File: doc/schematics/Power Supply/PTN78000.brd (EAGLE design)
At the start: 160 x 100 mm, 5 parts, among them U1 1.5APOWERMODULE

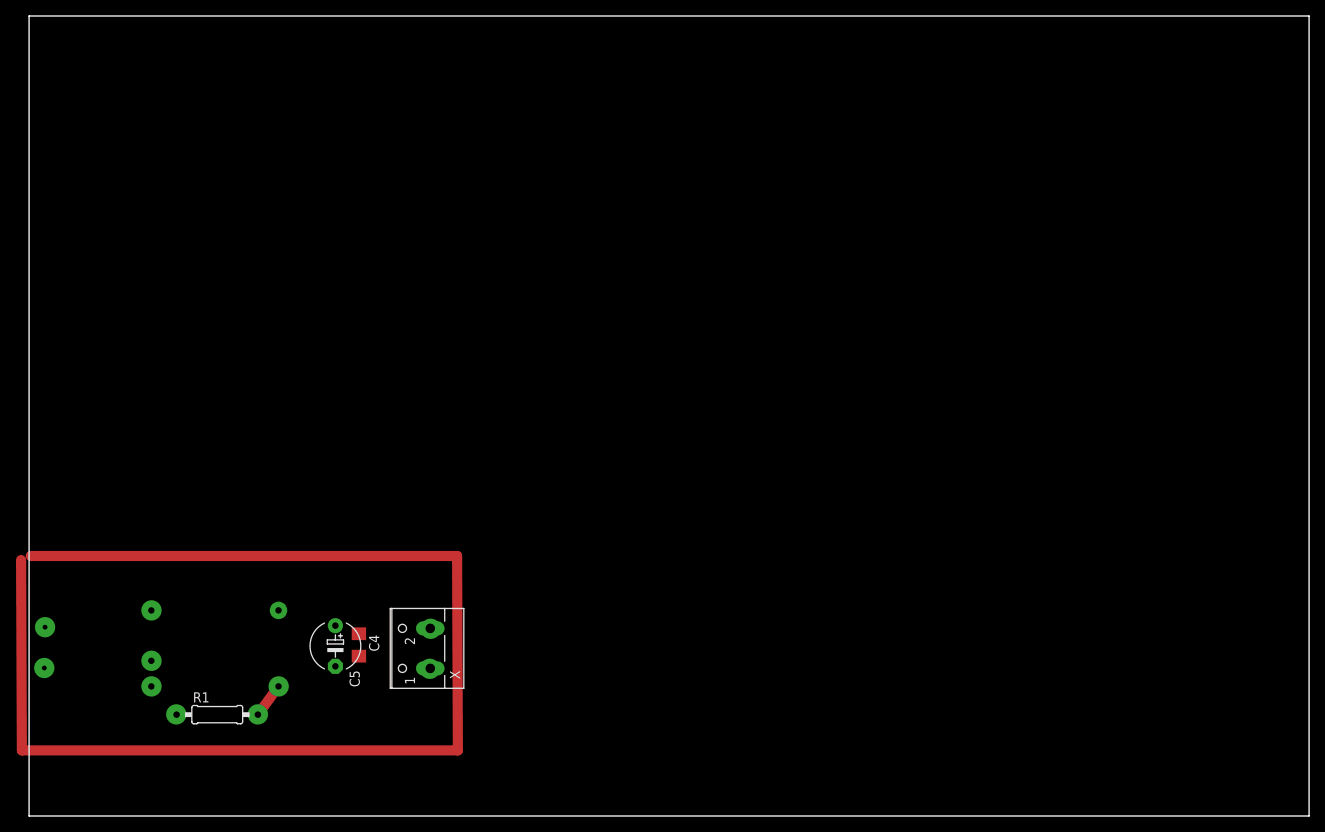
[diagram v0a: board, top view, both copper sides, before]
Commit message: New schematics
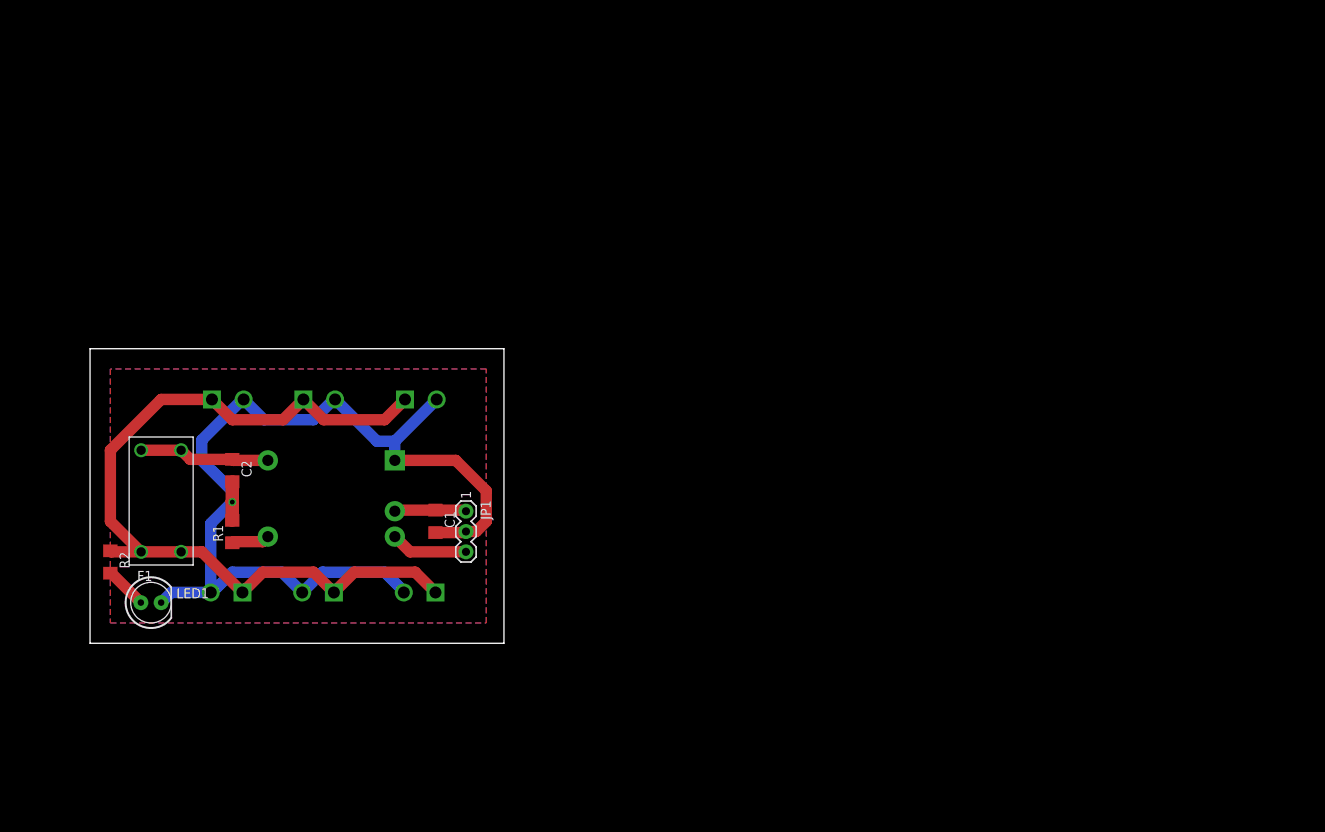
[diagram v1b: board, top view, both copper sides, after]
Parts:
- removed C4: (no value), rcl:C1206
- removed C5: (no value), rcl:E5-6
- removed U1: 1.5APOWERMODULE, TIPOWERMODULE:1.5APOWERMODULE
- removed X: OUTPUT (6 V), con-wago-500:W237-102
- added C1: 2.2 uF, ASL:1206
- added C2: 100 uF, ASL:1206
- added F1: FUSE, ASL:FUSE_2AG
- added J11, J13, J14, J15, J16, J9: POW_CONNECTFEMALE-RA, ASL:SOCKET-FEMALE_RA-3.96MM-2
- added JP1: M03PTH, ASL:1X03
- added LED1: (no value), SparkFun-LED:LED5MM
- added R2: 330, ASL:1206
- added U$1: PTN78000THROUGH-HOLE, ASL:PTN78000
- R1: value 13.1 K -> 21 K; device rcl:0207/10 -> ASL:1206
- moved R1 23.0 mm to (25.4, 35.6), turned to 90 degrees
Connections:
- removed net VCC: U1.P$2
- new net N$4: JP1.3, U$1.INHIBIT
- new net N$5: C2.1, F1.P$1, F1.P$2, U$1.V_OUT
- new net N$6: LED1.A, R2.2
- new net VCC5V0: F1.P$3, F1.P$4, J11.1, J13.1, J14.1, J15.1, J16.1, J9.1, R2.1
- net GND: now also C1.2, C2.2, J11.2, J13.2, J14.2, J15.2, J16.2, J9.2, JP1.2, LED1.K, R1.2, U$1.GND; no longer C4.2, C5.-, R1.1, U1.P$1
- net N$1: now also C1.1, JP1.1, U$1.V_IN; no longer R1.2, U1.P$4
- net N$2: now also R1.1, U$1.ADJ; no longer C4.1, C5.+, U1.P$5, X.2
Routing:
- net N$3: track 155.9 -> 0.00 mm
- net GND: track 0.00 -> 128.2 mm, vias 0 -> 1
- net VCC5V0: track 0.00 -> 105.0 mm
- net N$5: track 0.00 -> 16.4 mm, vias 1 -> 0
- net N$4: track 0.00 -> 9.68 mm, vias 1 -> 0
- net N$6: track 0.00 -> 5.33 mm, vias 1 -> 0
- net N$2: track 0.00 -> 4.76 mm
- net N$1: track 4.37 -> 9.00 mm
- added copper zone on layer 16, net GND
- added copper zone on layer 1, net VCC5V0
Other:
- board size 160 x 100 mm -> 51.7 x 36.8 mm
